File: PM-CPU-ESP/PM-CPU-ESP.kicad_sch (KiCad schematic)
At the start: 8 parts, among them J1 Conn_01x12_Pin, J2 Conn_01x12_Pin, J3 Conn_02x08_Odd_Even

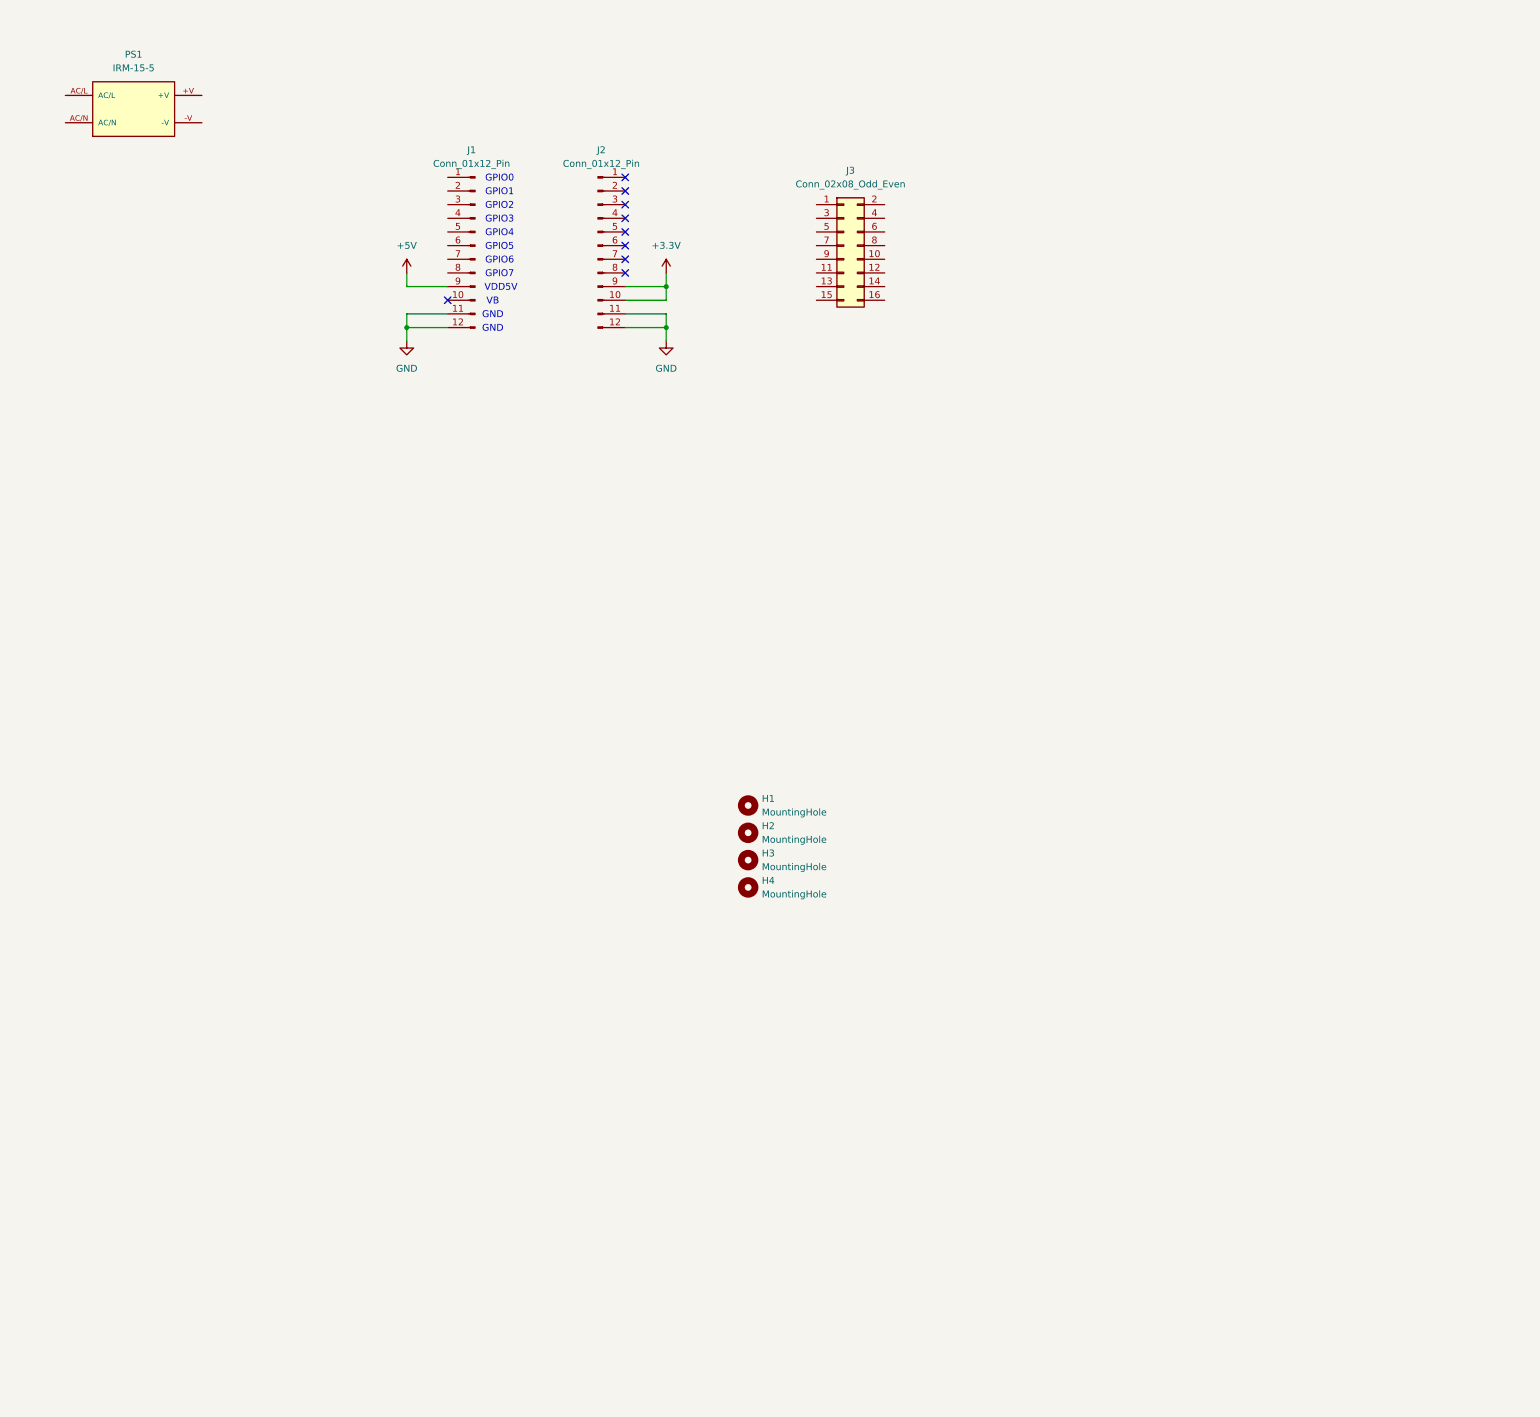
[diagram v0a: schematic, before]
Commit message: PM-CPU-ESP-front
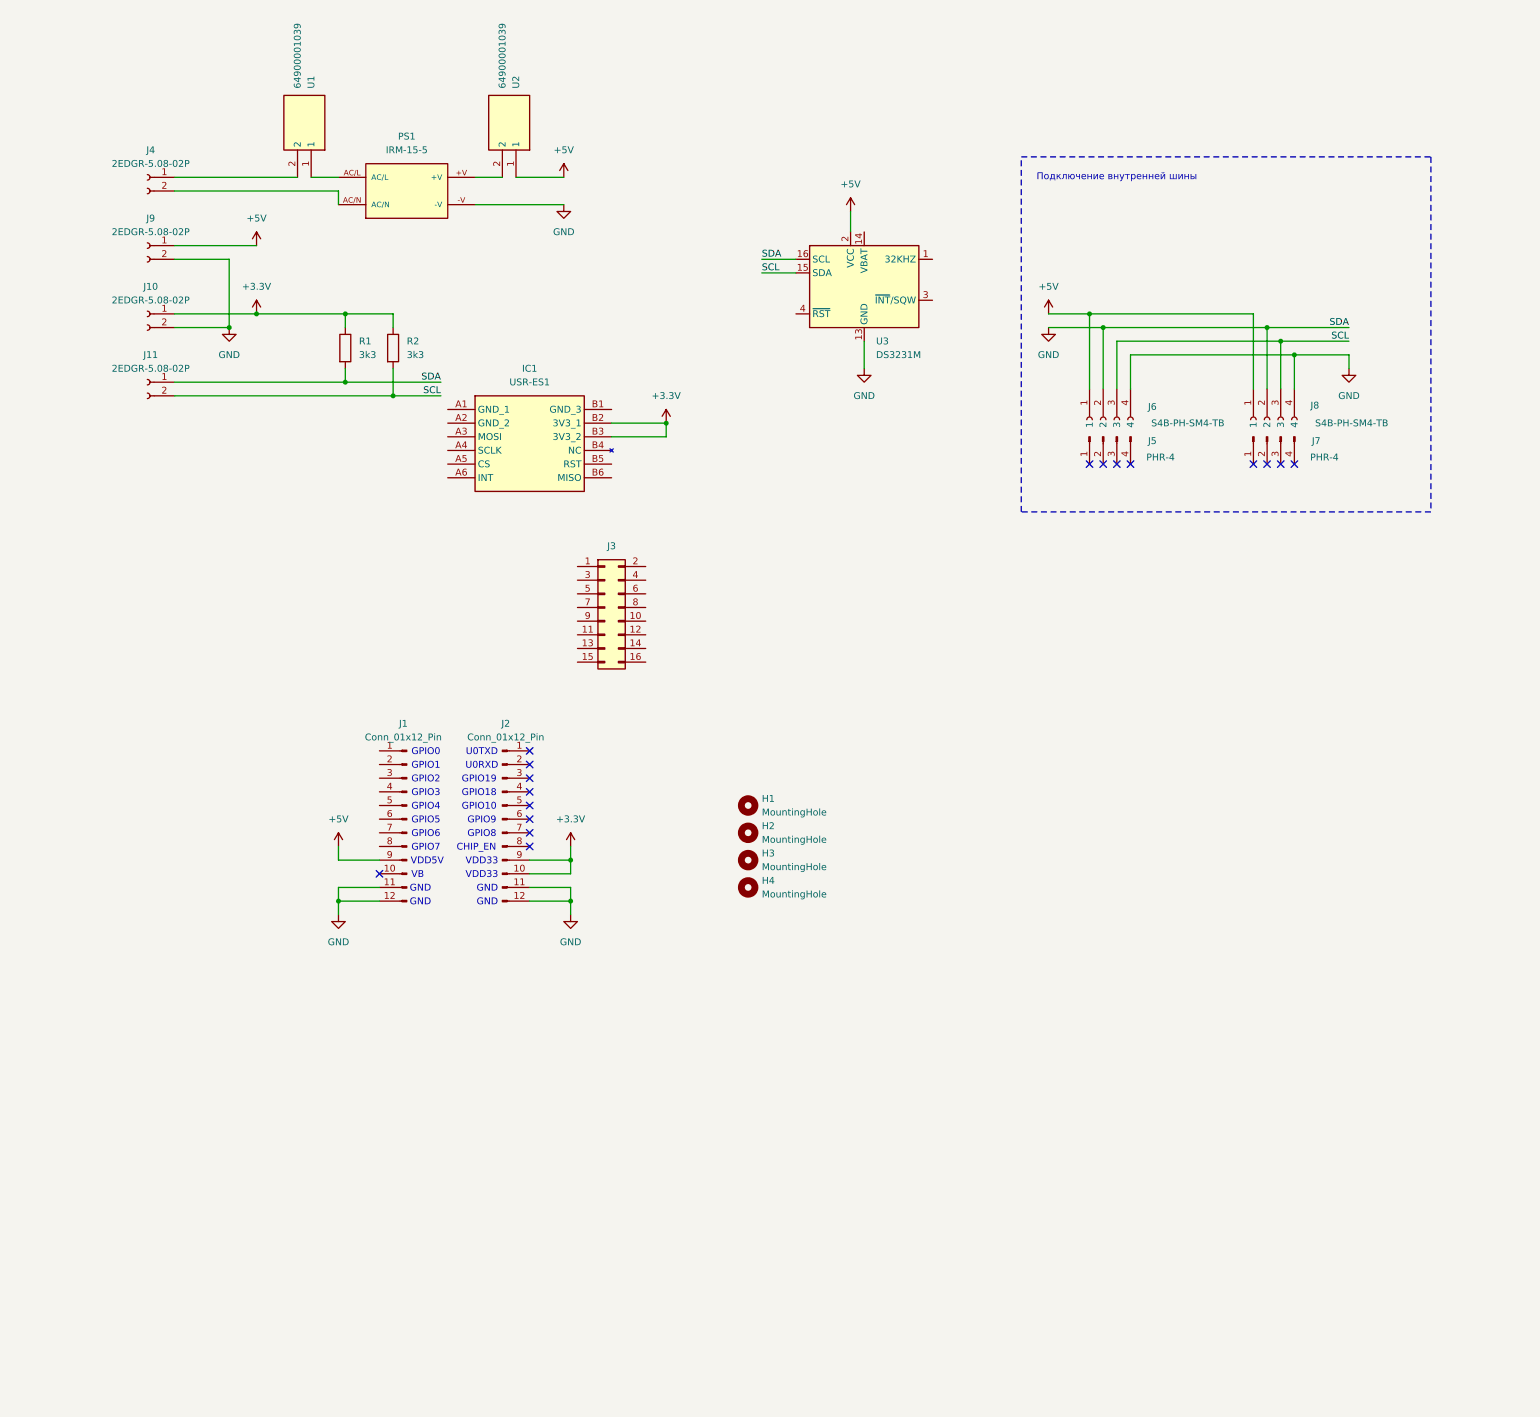
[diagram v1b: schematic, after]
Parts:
- removed J3: Conn_02x08_Odd_Even, Connector_PinSocket_2.54mm:PinSocket_2x08_P2.54mm_Vertical_SMD, symbol Connector_Generic:Conn_02x08_Odd_Even
- added IC1: USR-ES1, NextPCB:USRES1, symbol NextPCB:USR-ES1
- added J10, J11, J4, J9: 2EDGR-5.08-02P, NextPCB:Degson_2EDGR-5.08-02P, symbol NextPCB:Degson_2EDGR-5.08-02P
- added J3: Conn_02x08_socket, Connector_PinSocket_2.54mm:PinSocket_2x08_P2.54mm_Vertical_SMD, symbol NextPCB:Conn_02x08_socket
- added J5, J7: PHR-4, symbol NextPCB:JST_PHR-4
- added J6, J8: S4B-PH-SM4-TB, NextPCB:JST_S4B-PH-SM4-TB_JST_S4B-PH-SM4-TB, symbol NextPCB:JST_S4B-PH-SM4-TB
- added R1, R2: 3k3, Resistor_SMD:R_1206_3216Metric_Pad1.30x1.75mm_HandSolder, symbol NextPCB:R_3k3_0.25W
- added U1, U2: 64900001039, NextPCB:Fuseholder, symbol NextPCB:Fuseholder
- added U3: DS3231M, Package_SO:SOIC-16W_7.5x10.3mm_P1.27mm, symbol Timer_RTC:DS3231M
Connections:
- net +3.3V: now also IC1.B2 (3V3_1), IC1.B3 (3V3_2), J10.1 (Pin_1), R1.1, R2.1
- net +5V: now also J6.1, J8.1, J9.1 (Pin_1), U2.1, U3.2 (VCC)
- net GND: now also PS1.-V, J10.2 (Pin_2), J11.1 (Pin_1), J6.2, J6.4, J8.2, J8.4, J9.2 (Pin_2), R1.2, U3.10 (GND), U3.11 (GND), U3.12 (GND), U3.13 (GND), U3.16 (SCL), U3.5 (GND), U3.6 (GND), U3.7 (GND), U3.8 (GND), U3.9 (GND)
- net at PS1.+V: now also U2.2
- net at PS1.AC/L: now also U1.1
- net at PS1.AC/N: now also J4.2 (Pin_2)
- new net: J4.1 (Pin_1), U1.2
- new net SCL: J11.2 (Pin_2), J6.3, J8.3, R2.2, U3.15 (SDA)
- no-connect marks 9 -> 17
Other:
- note added: "CHIP_EN"
- note added: "GPIO10"
- note added: "GPIO18"
- note added: "GPIO19"
- note added: "GPIO8"
- note added: "GPIO9"
- note added: "U0RXD"
- note added: "U0TXD"
- note added: "VDD33"
- note added: "Подключение внутренней шины"
- moved on the sheet: J1, J2, PS1

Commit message: PM-CPU-ESP
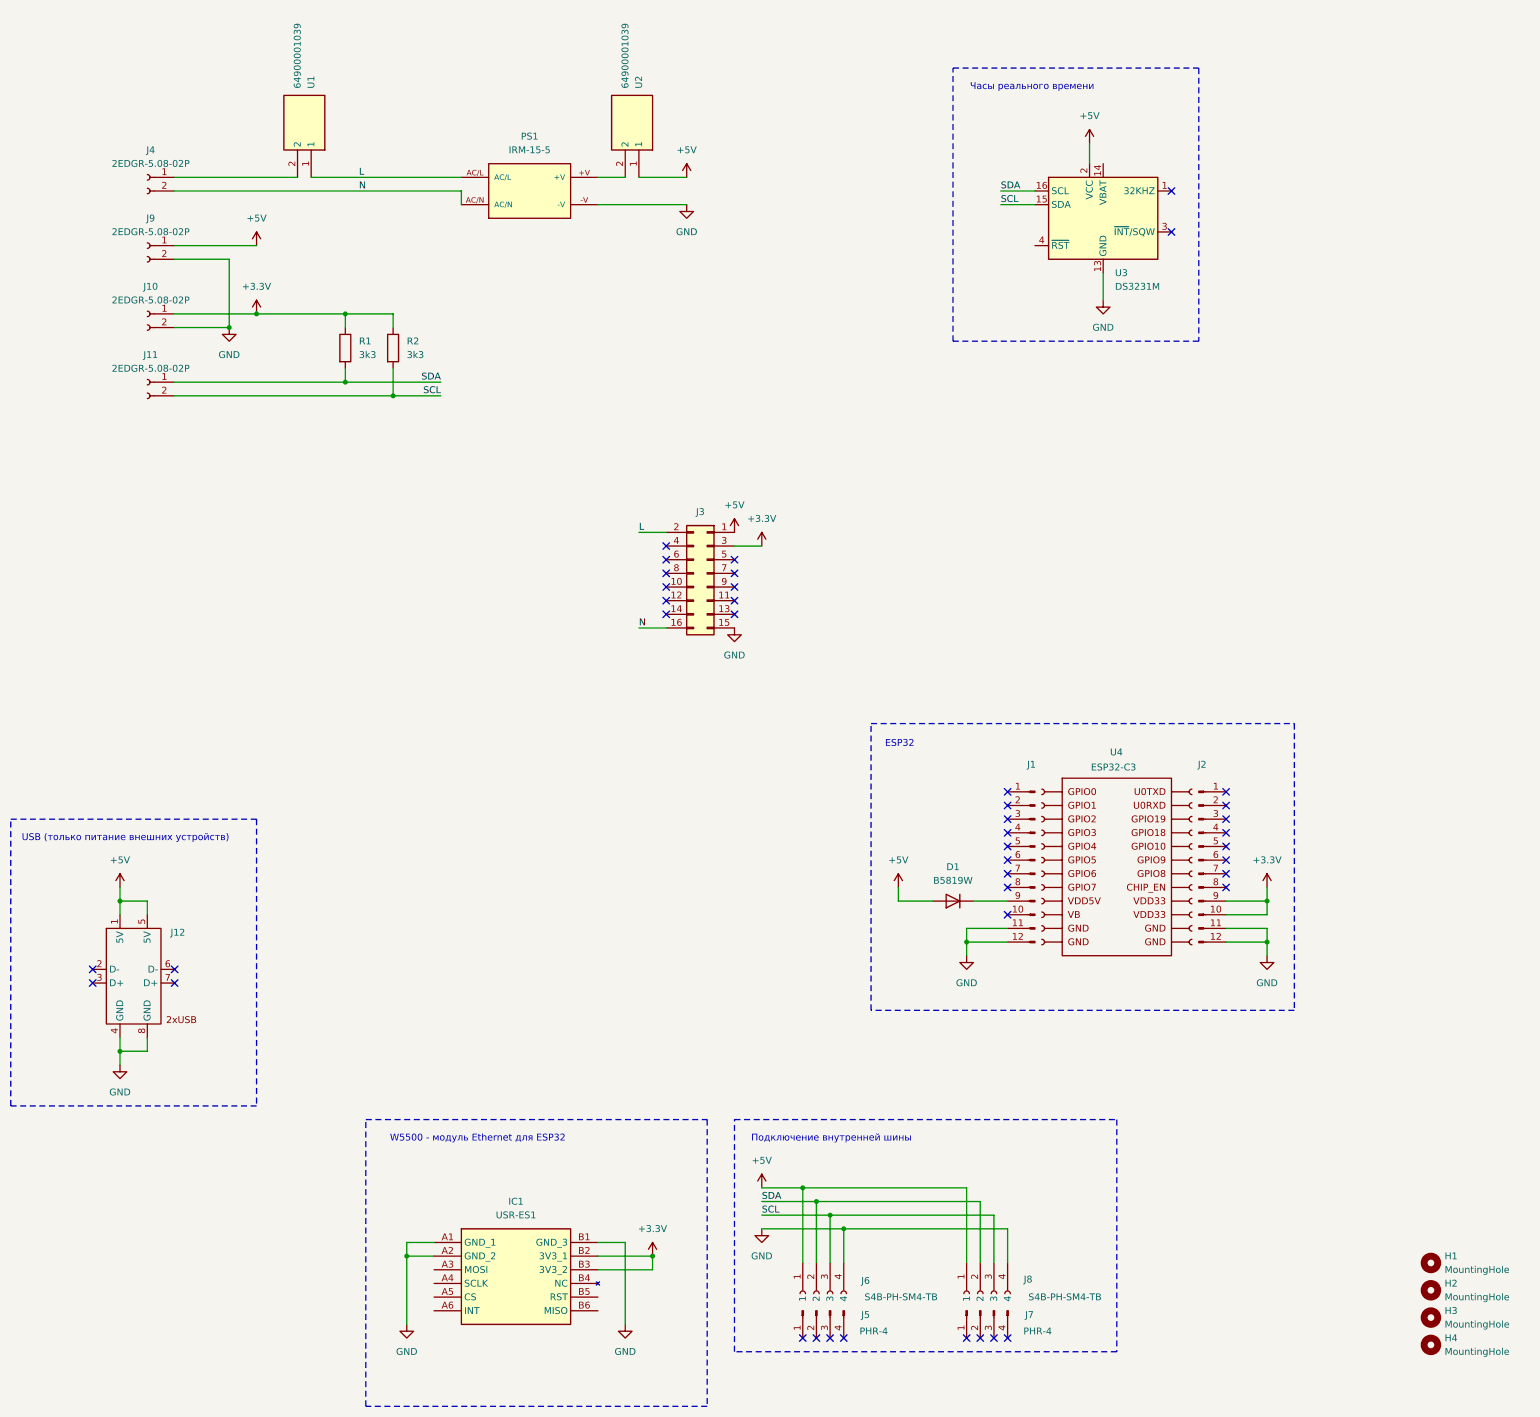
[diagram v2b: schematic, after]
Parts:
- added D1: B5819W, Diode_SMD:D_SOD-123, symbol NextPCB:B5819W
- added J12: ~, NextPCB:XKB_U224-08XN-1WR61, symbol NextPCB:XKB_U224-08XN-1WR61
- added U4: ESP32-C3, symbol NextPCB:Weact_Esp32-C3
- IC1: NextPCB_price (none) -> 4; NextPCB_url (none) -> https://aliexpress.ru/item/1005004860988013.html?spm=a2g2w.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
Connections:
- net +3.3V: now also J3.3 (Pin_3)
- net +5V: now also J3.1 (Pin_1), D1.2 (A), J12.1 (5V), J12.5 (5V); no longer J1.9 (Pin_9)
- net GND: now also IC1.A1 (GND_1), IC1.A2 (GND_2), IC1.B1 (GND_3), J3.15 (Pin_15), J12.4 (GND), J12.8 (GND); no longer J11.1 (Pin_1), J6.2, J8.2, R1.2, U3.16 (SCL)
- net N: now reaches J3.16 (Pin_16)
- net N: now also J4.2 (Pin_2), PS1.AC/N
- net L: now reaches J3.2 (Pin_2)
- net L: now also PS1.AC/L, U1.1
- new net: D1.1 (K), J1.9 (Pin_9)
- new net SDA: J11.1 (Pin_1), J6.2, J8.2, R1.2, U3.16 (SCL)
- no-connect marks 17 -> 42
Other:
- note added: "ESP32"
- note added: "USB (только питание внешних устройств)"
- note added: "W5500 - модуль Ethernet для ESP32"
- note added: "Часы реального времени"
- note removed: "CHIP_EN"
- note removed: "GND"
- note removed: "GPIO0"
- note removed: "GPIO1"
- note removed: "GPIO10"
- note removed: "GPIO18"
- note removed: "GPIO19"
- note removed: "GPIO2"
- note removed: "GPIO3"
- note removed: "GPIO4"
- note removed: "GPIO5"
- note removed: "GPIO6"
- note removed: "GPIO7"
- note removed: "GPIO8"
- note removed: "GPIO9"
- note removed: "U0RXD"
- note removed: "U0TXD"
- note removed: "VB"
- note removed: "VDD33"
- note removed: "VDD5V"
- moved on the sheet: H1, H2, H3, H4, IC1, J1, J2, J3, J5, J6, J7, J8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
